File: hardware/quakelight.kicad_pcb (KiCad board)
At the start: 4 copper layers, 40 x 62 mm, 85 parts, among them J1 USB_C_Receptacle_USB2.0, J10 Conn_01x02_MountingPin, J2 RJ45_Abracon_ARJP11A-MASA-B-A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, J3 EZmate-4, J4 PH, J5 PH, J7 TC2030-IDC-NL, J9 PH, SW1 SW_Push, SW2 SW_Push, U1 TPS7A0333DBVR, U10 STM32H573RIVx, U3 KSZ8081RNA, U4 SN74LVC2T45DCUR, U5 SN74LVC2T45DCUR, U6 TPS2116DRL, U8 SN74LVC2T45DCUR, Y1 25MHz, Y2 32.768kHz

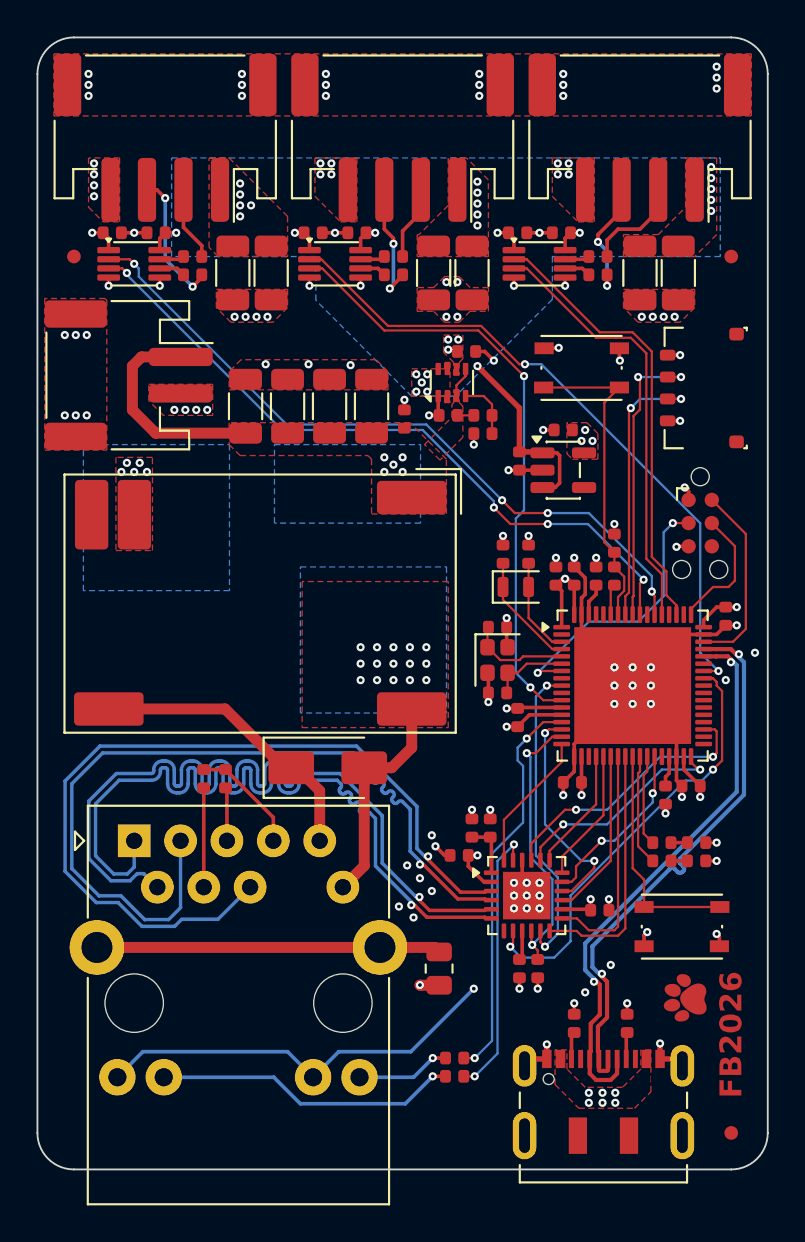
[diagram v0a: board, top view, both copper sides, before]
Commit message: wip
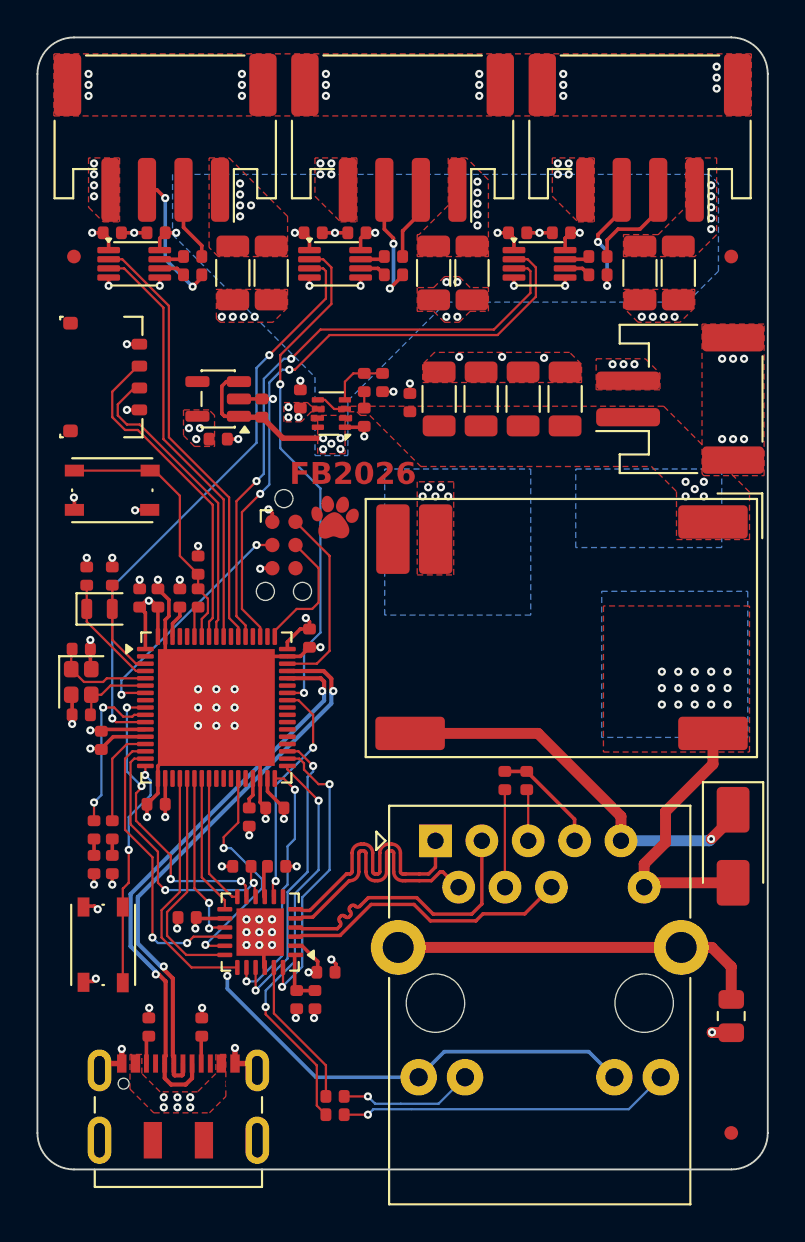
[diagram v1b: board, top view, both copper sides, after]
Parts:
- moved J3 33.1 mm to (123.5, 98.6), turned to -90 degrees
- moved R21 33.0 mm to (123.1, 125.3), turned to -90 degrees
- moved G*** 32.6 mm to (136.3, 106.3), turned to 0 degrees
- moved R4 32.0 mm to (124.1, 125.3), turned to -90 degrees
- moved SW2 31.7 mm to (123.6, 129.7), turned to -90 degrees
- moved D2 31.1 mm to (123.1, 123.4), turned to 90 degrees
- moved J10 30.2 mm to (155.2, 99.8), turned to 90 degrees
- moved D1 30.1 mm to (124.1, 123.4), turned to 90 degrees
- moved SW1 26.6 mm to (124.1, 104.8), turned to 0 degrees
- moved R1 23.3 mm to (129.0, 134.2)
- moved R2 23.3 mm to (126.1, 134.2)
- moved J1 23.3 mm to (127.7, 139.2)
- moved C17 22.8 mm to (123.5, 118.5)
- moved C11 22.8 mm to (124.1, 109.5)
- moved C58 22.8 mm to (131.6, 122.7)
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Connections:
- U10 pad 10: unconnected-(U10-PC2-Pad10) -> /LED_B
- U10 pad 14: /ETH_LED_0 -> /LED_A
- U10 pad 17: /ETH_RESET -> /SW0
- U10 pad 26: /SW0 -> unconnected-(U10-PB0-Pad26)
- U10 pad 27: /LED_B -> unconnected-(U10-PB1-Pad27)
- U10 pad 28: /LED_A -> unconnected-(U10-PB2-Pad28)
- U10 pad 35: unconnected-(U10-PB13-Pad35) -> /ETH_LED_0
- U10 pad 36: unconnected-(U10-PB14-Pad36) -> /ETH_RESET
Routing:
- net /ETH_TX_P: track 45.8 -> 15.5 mm, vias 1 -> 0
- net /ETH_RX_N: track 46.2 -> 15.9 mm, vias 1 -> 0
- net /ETH_RX_P: track 46.1 -> 15.8 mm, vias 1 -> 0
- net /ETH_TX_N: track 45.9 -> 15.7 mm, vias 1 -> 0
- net /SPI1_MOSI: track 38.6 -> 23.3 mm, vias 4 -> 0
- net /SPI1_SCK: track 39.4 -> 24.0 mm, vias 4 -> 0
- net Net-(J2-Pad14): track 5.14 -> 18.2 mm
- net +5V_DCDC: track 14.6 -> 2.59 mm
- net /MCO1: track 23.9 -> 12.6 mm
- net /SPI3_SCK: track 24.6 -> 34.5 mm, vias 0 -> 2
- net /SPI3_MOSI: track 23.8 -> 33.6 mm, vias 0 -> 2
- net Net-(J2-Pad12): track 16.7 -> 7.39 mm
- net /ETH_RESET: track 7.67 -> 16.4 mm, vias 0 -> 2
- net /SPI2_SCK: track 36.7 -> 28.0 mm
- net /RMII_TX_EN: track 6.73 -> 14.0 mm
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
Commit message: wip
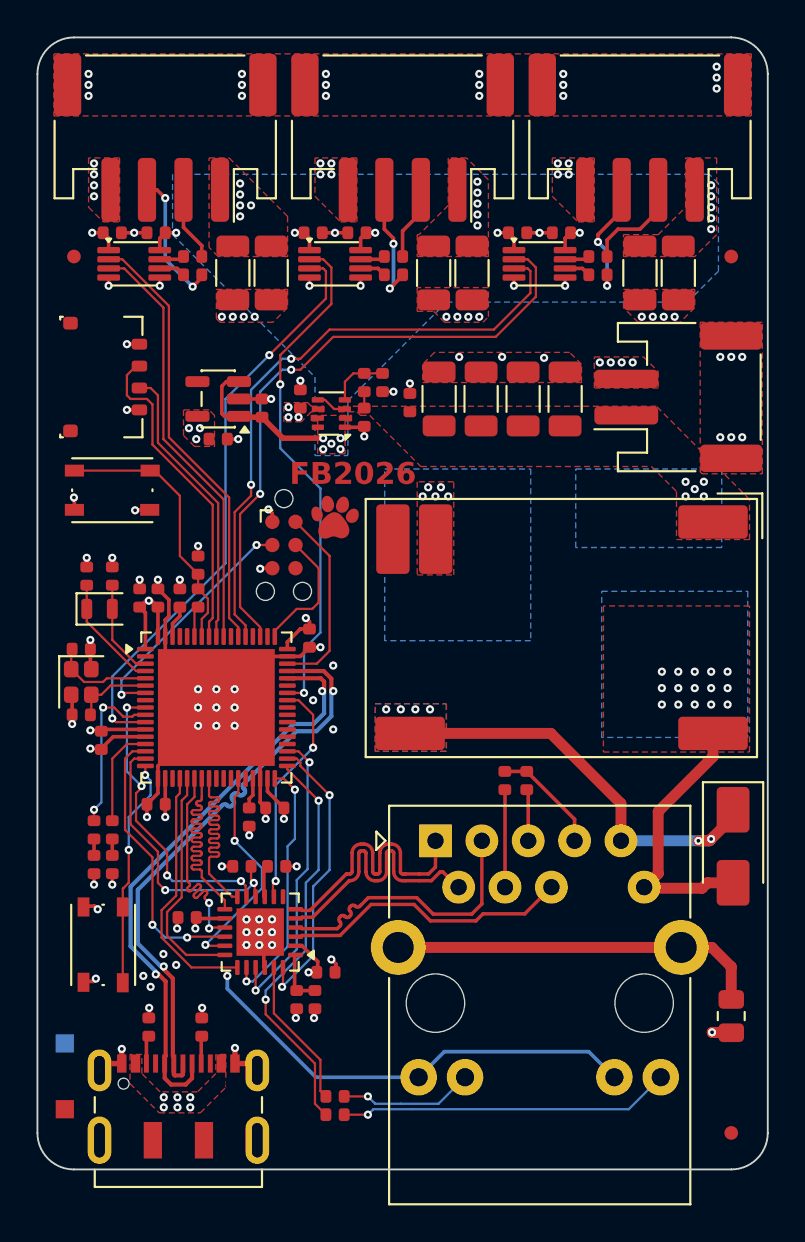
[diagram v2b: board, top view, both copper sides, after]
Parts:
- added REF**: 4layer-flags-line, balto:4layer-flags-line, F.Cu at (121.5, 136.9)
- moved J10 0.14 mm to (155.1, 99.7)
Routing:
- net /RMII_RXD0: track 7.69 -> 14.5 mm
- net /RMII_RXD1: track 7.29 -> 13.7 mm
- net /RMII_CRS_DV: track 9.43 -> 12.1 mm
- net /USB_D+: track 30.8 -> 32.4 mm
- net /UART_TX: track 17.0 -> 15.8 mm
- net /POE_V+: track 21.9 -> 23.0 mm, vias 1 -> 6
- net /RMII_RX_ER: track 12.9 -> 12.2 mm
- net /RMII_REF_CLK: track 15.9 -> 15.3 mm
- net /USB_D-: track 31.8 -> 32.4 mm
- net GND: track 72.9 -> 72.8 mm, vias 118 -> 126
- added copper zone on B.Cu, net /POE_V+
- added copper zone on F.Cu, net /POE_V+
